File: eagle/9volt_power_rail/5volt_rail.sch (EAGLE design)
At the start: 32 parts, among them X1 5566-4, X2 5566-4, X3 5566-4, X4 5566-4, X5 5566-4, X6 5566-4

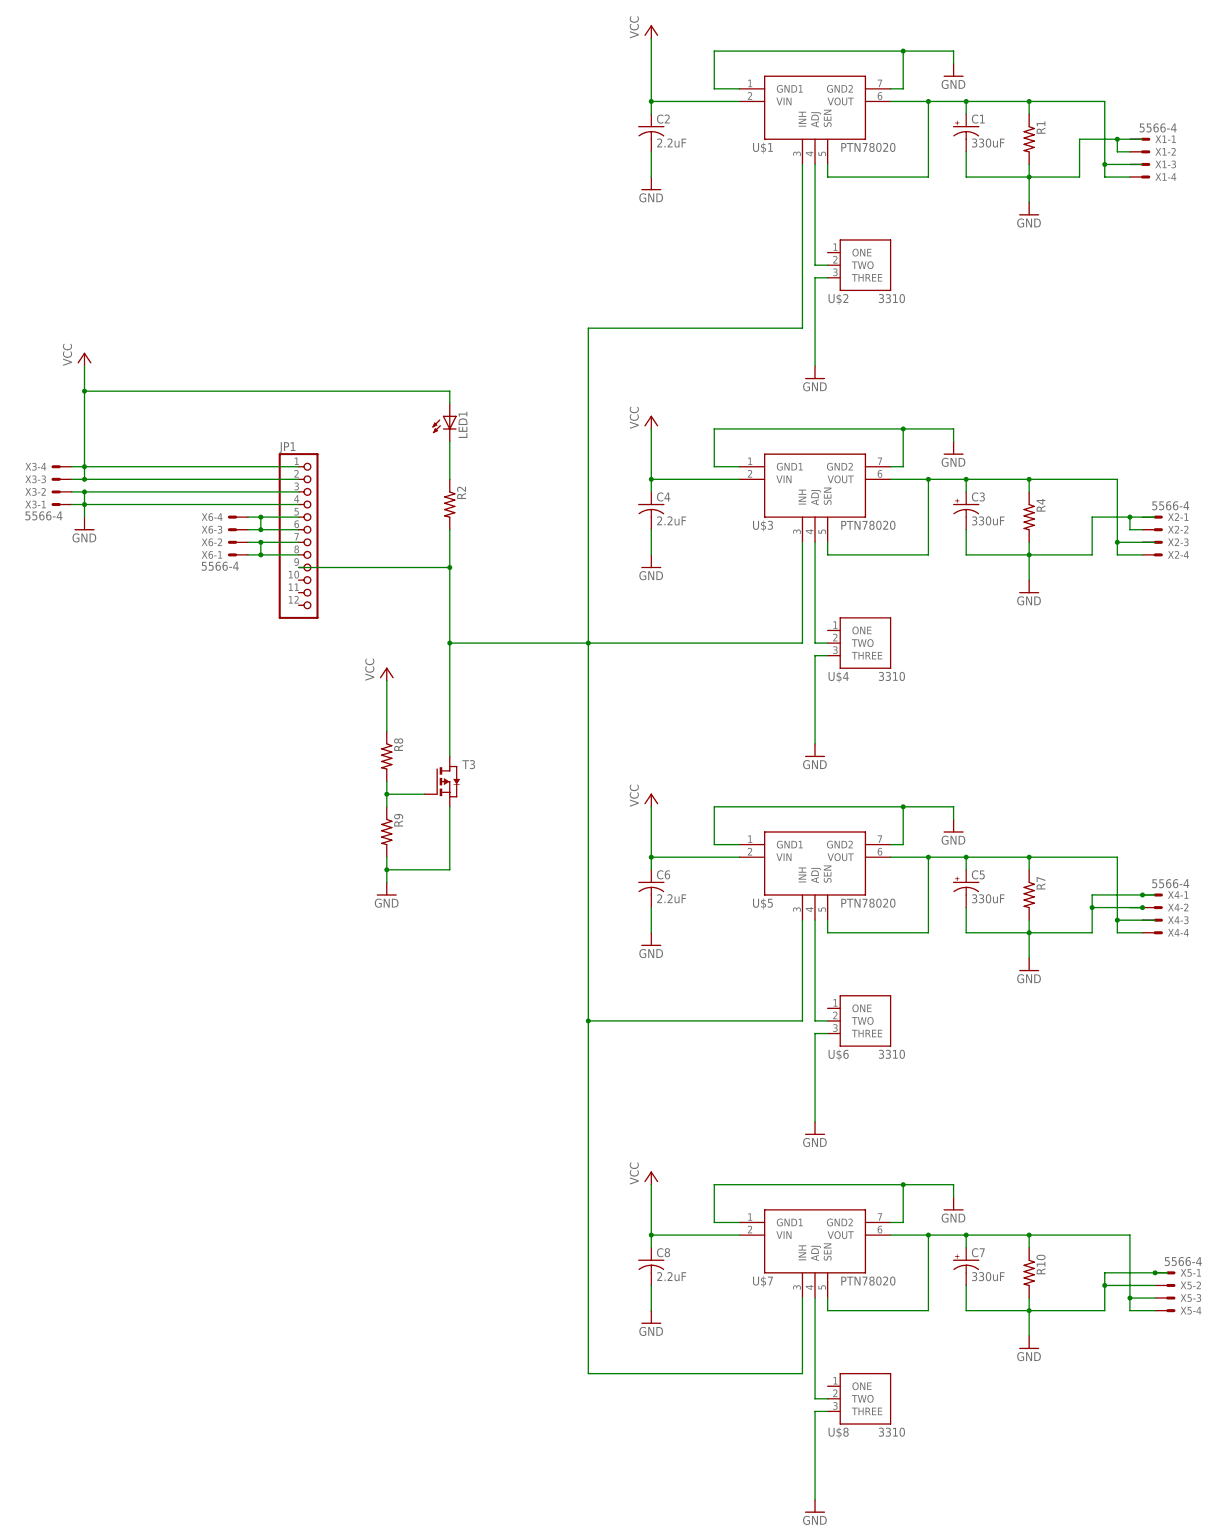
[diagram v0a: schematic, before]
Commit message: moving to lab computer
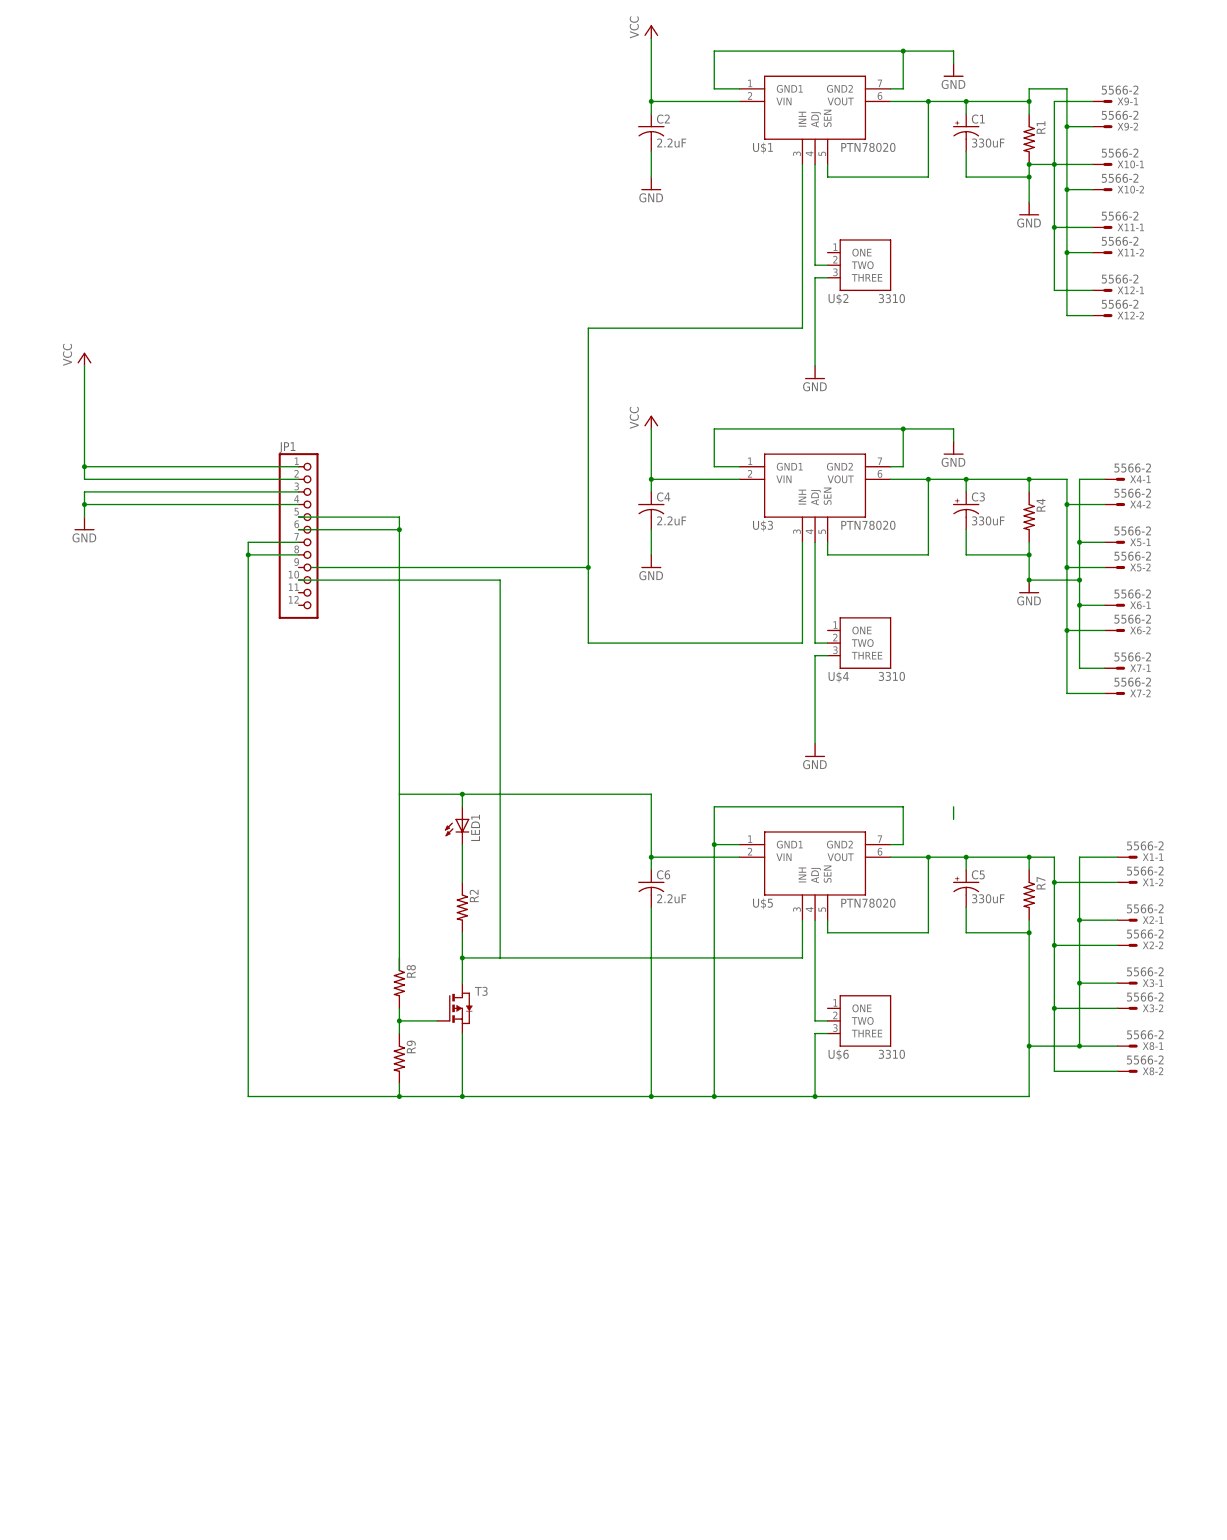
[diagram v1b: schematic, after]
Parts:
- removed C7: 330uF, rcl:CPOL-USE5-10.5
- removed C8: 2.2uF, adafruit:C-USC0805
- removed R10: (no value), adafruit:R-US_M0805
- removed U$7: PTH78020-SMD, PTN78020:PTH78020-SMD
- removed U$8: 3310-001, 3310-001:3310-001
- added X10, X11, X12, X7, X8, X9: 5566-2, con-molex:5566-2
- X1, X2, X3, X4, X5, X6: value 5566-4 -> 5566-2; device con-molex:5566-4 -> con-molex:5566-2
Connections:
- removed net N$1: C3.+, R4.1, U$3.SEN, U$3.VOUT, X2-4.S
- removed net N$10: JP1.7, JP1.8, X6-1.S, X6-2.S
- removed net N$22: U$7.ADJ, U$8.TWO
- removed net N$3: C1.+, R1.1, U$1.SEN, U$1.VOUT, X1-4.S
- removed net N$5: JP1.9, R2.2, T3.D, U$1.INH, U$3.INH, U$5.INH, U$7.INH
- removed net N$6: C5.+, R7.1, U$5.SEN, U$5.VOUT, X4-3.S, X4-4.S
- new net N$11: C6.1, JP1.5, JP1.6, LED1.A, U$5.VIN
- new net N$13: C3.+, R4.1, U$3.SEN, U$3.VOUT, X4-2.S, X5-2.S, X6-2.S, X7-2.S
- new net N$15: C5.+, R7.1, U$5.SEN, U$5.VOUT, X1-2.S, X2-2.S, X3-2.S, X8-2.S
- new net N$19: C5.-, C6.2, JP1.7, JP1.8, R7.2, R9.2, T3.S, U$5.GND1, U$5.GND2, U$6.THREE, X1-1.S, X2-1.S, X3-1.S, X8-1.S
- new net N$8: C1.+, R1.1, U$1.SEN, U$1.VOUT, X10-2.S, X11-2.S, X12-2.S, X9-2.S
- net GND: now also X10-1.S, X11-1.S, X12-1.S, X6-1.S, X7-1.S, X9-1.S; no longer C5.-, C6.2, C7.-, C8.2, R10.2, R7.2, R9.2, T3.S, U$5.GND1, U$5.GND2, U$6.THREE, U$7.GND1, U$7.GND2, U$8.THREE, X1-2.S, X2-2.S, X3-1.S, X3-2.S, X4-2.S, X5-2.S
- net N$7: now also JP1.10, R2.2, T3.D, U$5.INH; no longer JP1.5, JP1.6, X6-3.S, X6-4.S
- net N$9: now also U$1.INH, U$3.INH; no longer C7.+, R10.1, U$7.SEN, U$7.VOUT, X5-3.S, X5-4.S
- net VCC: no longer C6.1, C8.1, LED1.A, R8.1, U$5.VIN, U$7.VIN, X3-3.S, X3-4.S
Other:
- moved on the sheet: LED1, R2, R8, R9, T3, X1-1, X1-2, X2-1, X2-2, X3-1, X3-2, X4-1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
